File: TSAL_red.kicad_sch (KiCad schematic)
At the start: 43 parts, among them Q7 NMOS, U1 OPA355NA, U17 TBA1-0511E, U4 SFH617A-1X007T, U5 NE555D

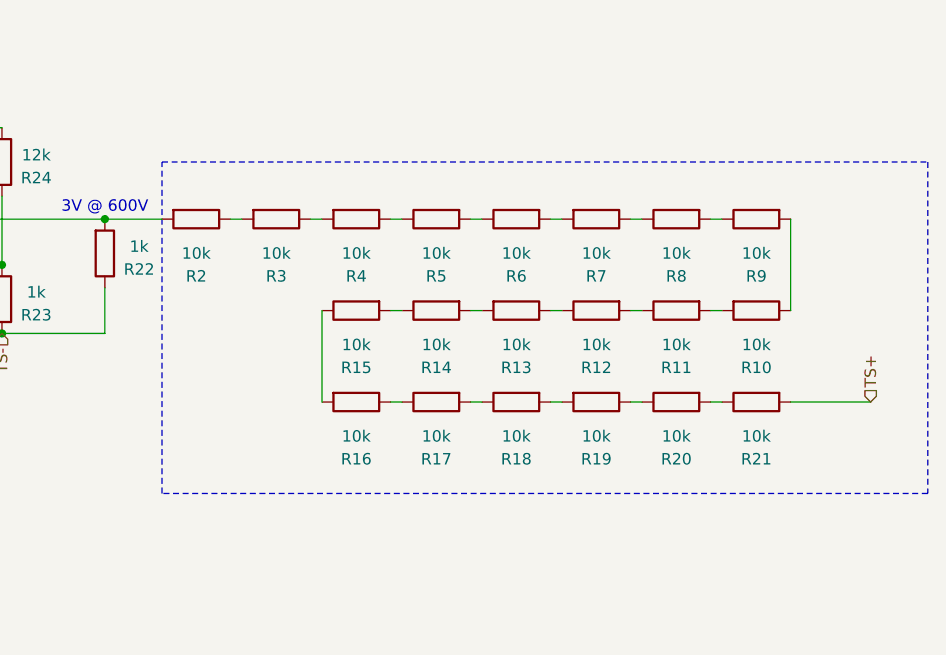
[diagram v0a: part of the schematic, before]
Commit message: Submission Ready. ESF 15.07.24
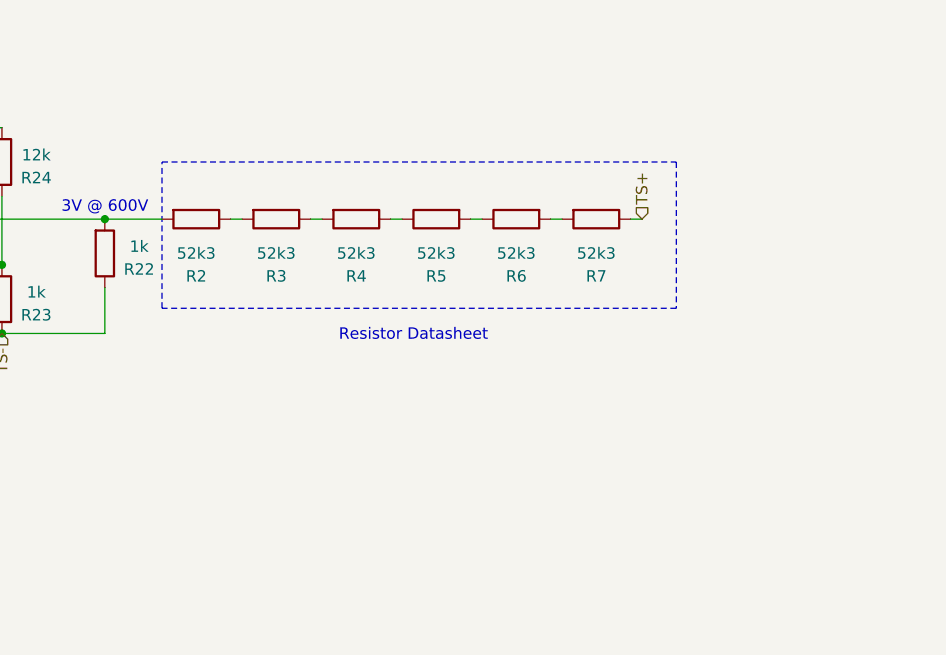
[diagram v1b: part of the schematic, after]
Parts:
- removed R10, R11, R12, R13, R14, R15, R16, R17, R18, R19, R20, R21, R8, R9: 10k, Resistor_SMD:R_0603_1608Metric, symbol Device:R
- R2, R3, R4, R5, R6, R7: value 10k -> 52k3; footprint Resistor_SMD:R_0603_1608Metric -> Resistor_SMD:R_0805_2012Metric; Cost (none) -> 0.05; Mouser (none) -> 603-RT0805DRD0752K3L
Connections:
- net TS+: now also R7.1
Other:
- note added: "Resistor Datasheet"
